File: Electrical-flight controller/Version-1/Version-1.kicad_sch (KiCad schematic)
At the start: 4 parts, among them U1 MPU-6050, U2 ATmega328P-A, U3 BMP280, U4 LM1117DT-ADJ

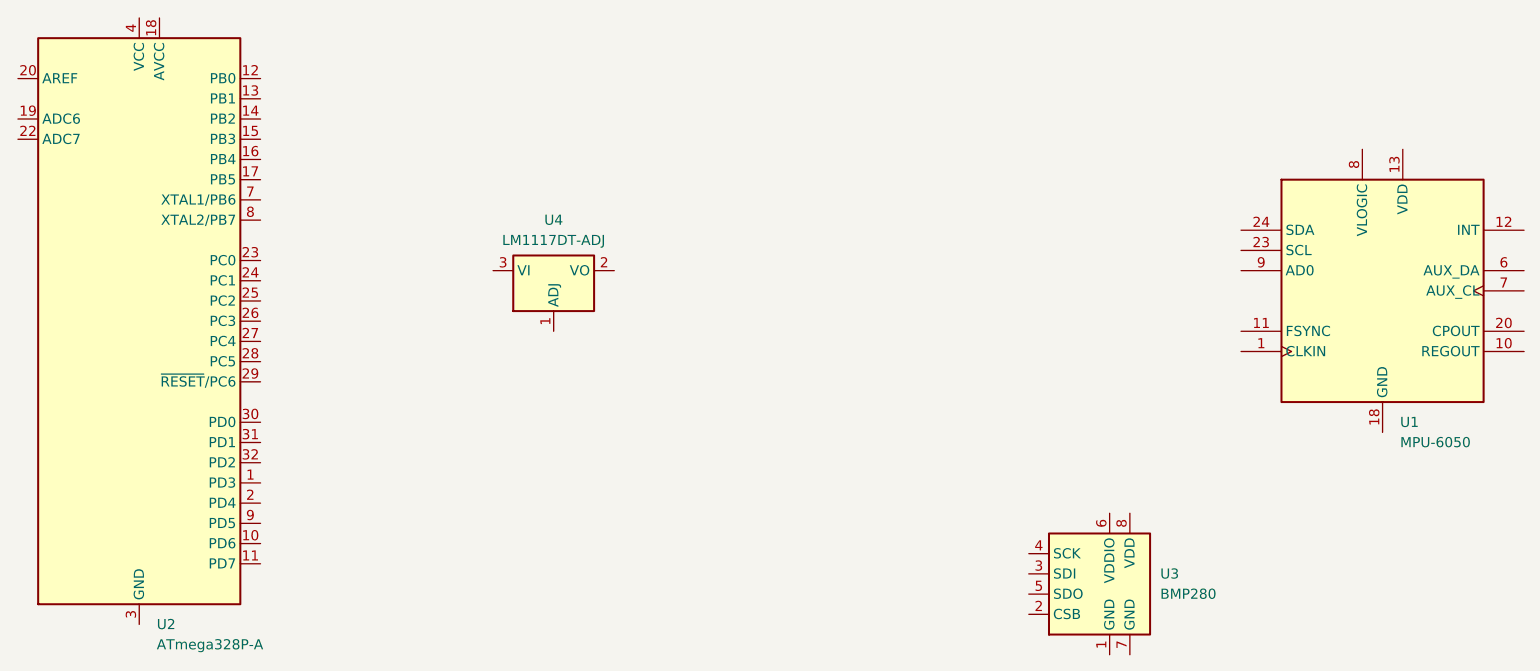
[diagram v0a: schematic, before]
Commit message: Started ESP32
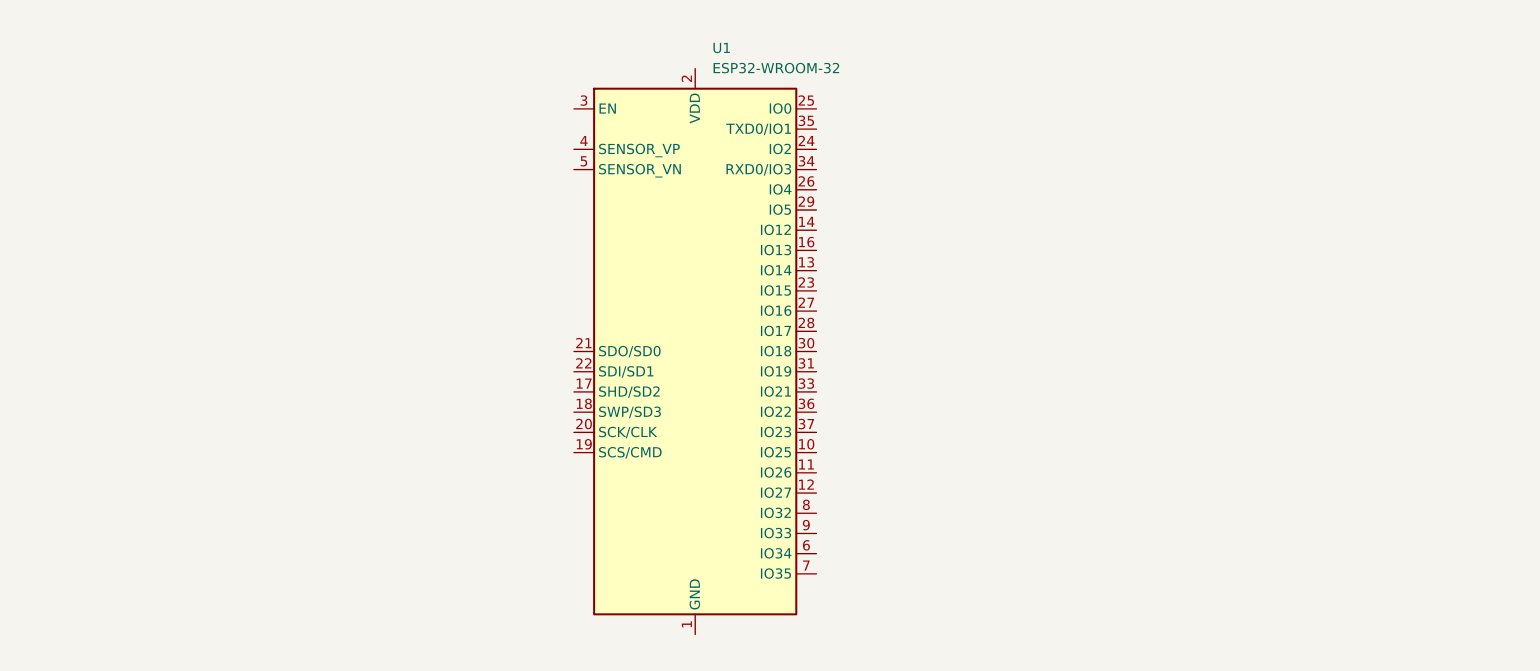
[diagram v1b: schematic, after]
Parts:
- removed U1: MPU-6050, Sensor_Motion:InvenSense_QFN-24_4x4mm_P0.5mm, symbol Sensor_Motion:MPU-6050
- removed U2: ATmega328P-A, Package_QFP:TQFP-32_7x7mm_P0.8mm, symbol MCU_Microchip_ATmega:ATmega328P-A
- removed U3: BMP280, Package_LGA:Bosch_LGA-8_2x2.5mm_P0.65mm_ClockwisePinNumbering, symbol Sensor_Pressure:BMP280
- removed U4: LM1117DT-ADJ, Package_TO_SOT_SMD:TO-252-3_TabPin2, symbol Regulator_Linear:LM1117DT-ADJ
- added U1: ESP32-WROOM-32, RF_Module:ESP32-WROOM-32, symbol RF_Module:ESP32-WROOM-32
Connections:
- new net: U1.1 (GND), U1.15 (GND), U1.38 (GND), U1.39 (GND)

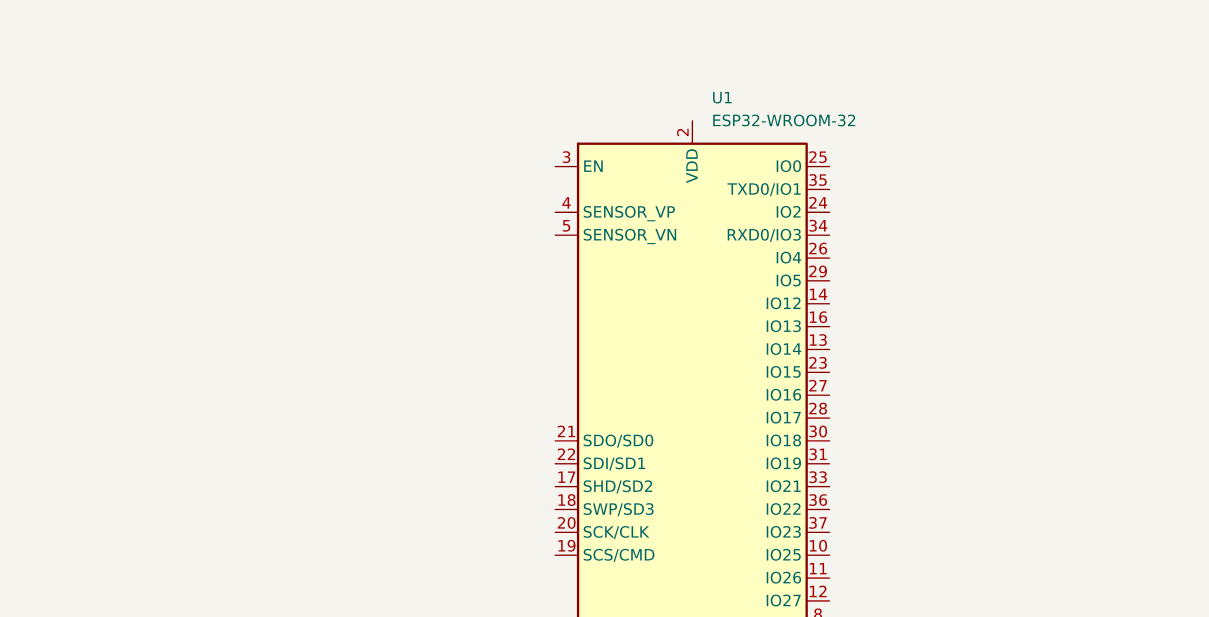
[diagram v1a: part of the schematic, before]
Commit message: 2nd update
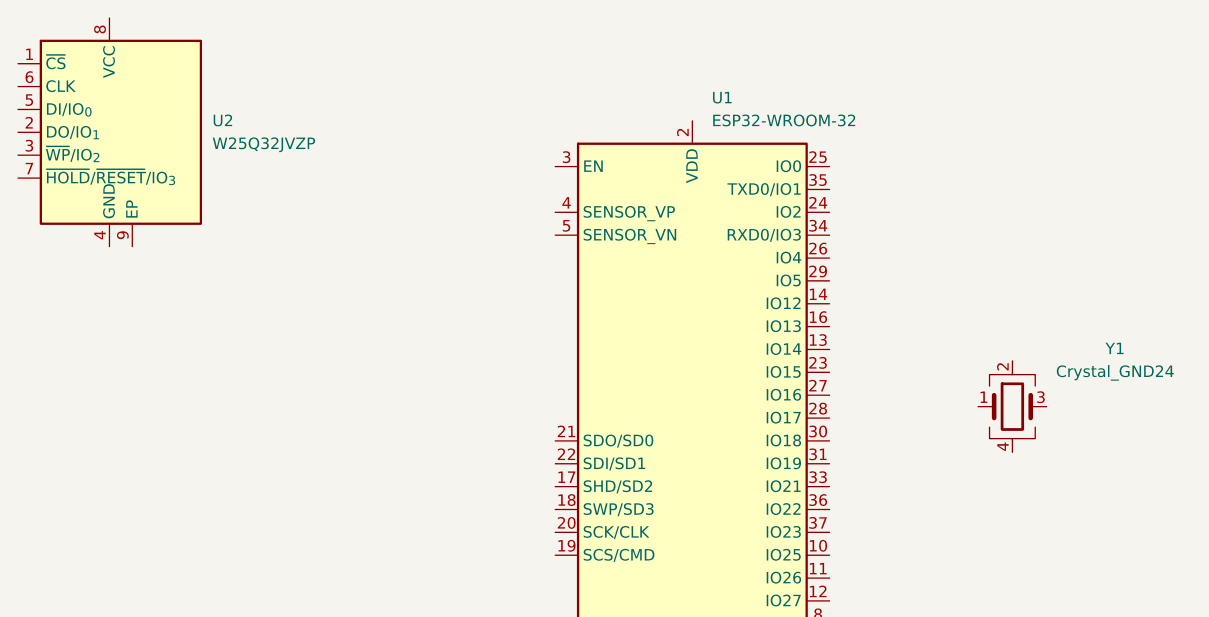
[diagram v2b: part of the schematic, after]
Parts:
- added U2: W25Q32JVZP, Package_SON:WSON-8-1EP_6x5mm_P1.27mm_EP3.4x4.3mm, symbol Memory_Flash:W25Q32JVZP
- added Y1: Crystal_GND24, symbol Device:Crystal_GND24
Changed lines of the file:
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@@
 	(paper "A4")
+	(symbol
+		(lib_id "Device:Crystal_GND24")
+		(at 170.18 78.74 0)
+		(unit 1)
+		(exclude_from_sim no)
+		(in_bom yes)
+		(on_board yes)
+		(dnp no)
+		(fields_autoplaced yes)
+		(property "Reference" "Y1"
+			(at 181.61 72.3198 0)
+			(effects
+				(font
+					(size 1.27 1.27)
+				)
+			)
+		)
+		(property "Value" "Crystal_GND24"
+			(at 181.61 74.8598 0)
+			(effects
+				(font
+					(size 1.27 1.27)
+				)
+			)
+		)
+		(property "Footprint" ""
+			(at 170.18 78.74 0)
+			(effects
+				(font
+					(size 1.27 1.27)
+				)
+				(hide yes)
+			)
+		)
+		(property "Datasheet" "~"
+			(at 170.18 78.74 0)
+			(effects
+				(font
+					(size 1.27 1.27)
+				)
+				(hide yes)
+			)
+		)
+		(property "Description" "Four pin crystal, GND on pins 2 and 4"
+			(at 170.18 78.74 0)
+			(effects
+				(font
+					(size 1.27 1.27)
+				)
+				(hide yes)
+			)
+		)
+		(pin "1"
+		)
+		(pin "2"
+		)
+		(pin "3"
+		)
+		(pin "4"
+		)
+		(instances
+			(project ""
+				(path "/b01821f6-bde1-4035-92df-fac2c021cb26"
+					(reference "Y1")
+					(unit 1)
+				)
+			)
+		)
+	)
+	(symbol
+		(lib_id "Memory_Flash:W25Q32JVZP")
+		(at 69.85 48.26 0)
+		(unit 1)
+		(exclude_from_sim no)
+		(in_bom yes)
+		(on_board yes)
+		(dnp no)
+		(fields_autoplaced yes)
+		(property "Reference" "U2"
+			(at 81.28 46.9899 0)
+			(effects
+				(font
+					(size 1.27 1.27)
+				)
+				(justify left)
+			)
+		)
+		(property "Value" "W25Q32JVZP"
+			(at 81.28 49.5299 0)
+			(effects
+				(font
+					(size 1.27 1.27)
+				)
+				(justify left)
+			)
+		)
+		(property "Footprint" "Package_SON:WSON-8-1EP_6x5mm_P1.27mm_EP3.4x4.3mm"
+			(at 69.85 48.26 0)
+			(effects
+				(font
+					(size 1.27 1.27)
+				)
+				(hide yes)
+			)
+		)
+		(property "Datasheet" "http://www.winbond.com/resource-files/w25q32jv%20revg%2003272018%20plus.pdf"
+			(at 69.85 50.8 0)
+			(effects
+				(font
+					(size 1.27 1.27)
+				)
+				(hide yes)
+			)
+		)
+		(property "Description" "32Mbit / 4MiB Serial Flash Memory, Standard/Dual/Quad SPI, 2.7-3.6V, WSON-8"
+			(at 69.85 48.26 0)
+			(effects
+				(font
+					(size 1.27 1.27)
+				)
+				(hide yes)
+			)
+		)
+		(pin "5"
+		)
+		(pin "7"
+		)
+		(pin "2"
+		)
+		(pin "9"
+		)
+		(pin "1"
+		)
+		(pin "6"
+		)
+		(pin "3"
+		)
+		(pin "8"
+		)
+		(pin "4"
+		)
+		(instances
+			(project ""
+				(path "/b01821f6-bde1-4035-92df-fac2c021cb26"
+					(reference "U2")
+					(unit 1)
+				)
+			)
+		)
+	)
 	(symbol
 		(lib_id "RF_Module:ESP32-WROOM-32")

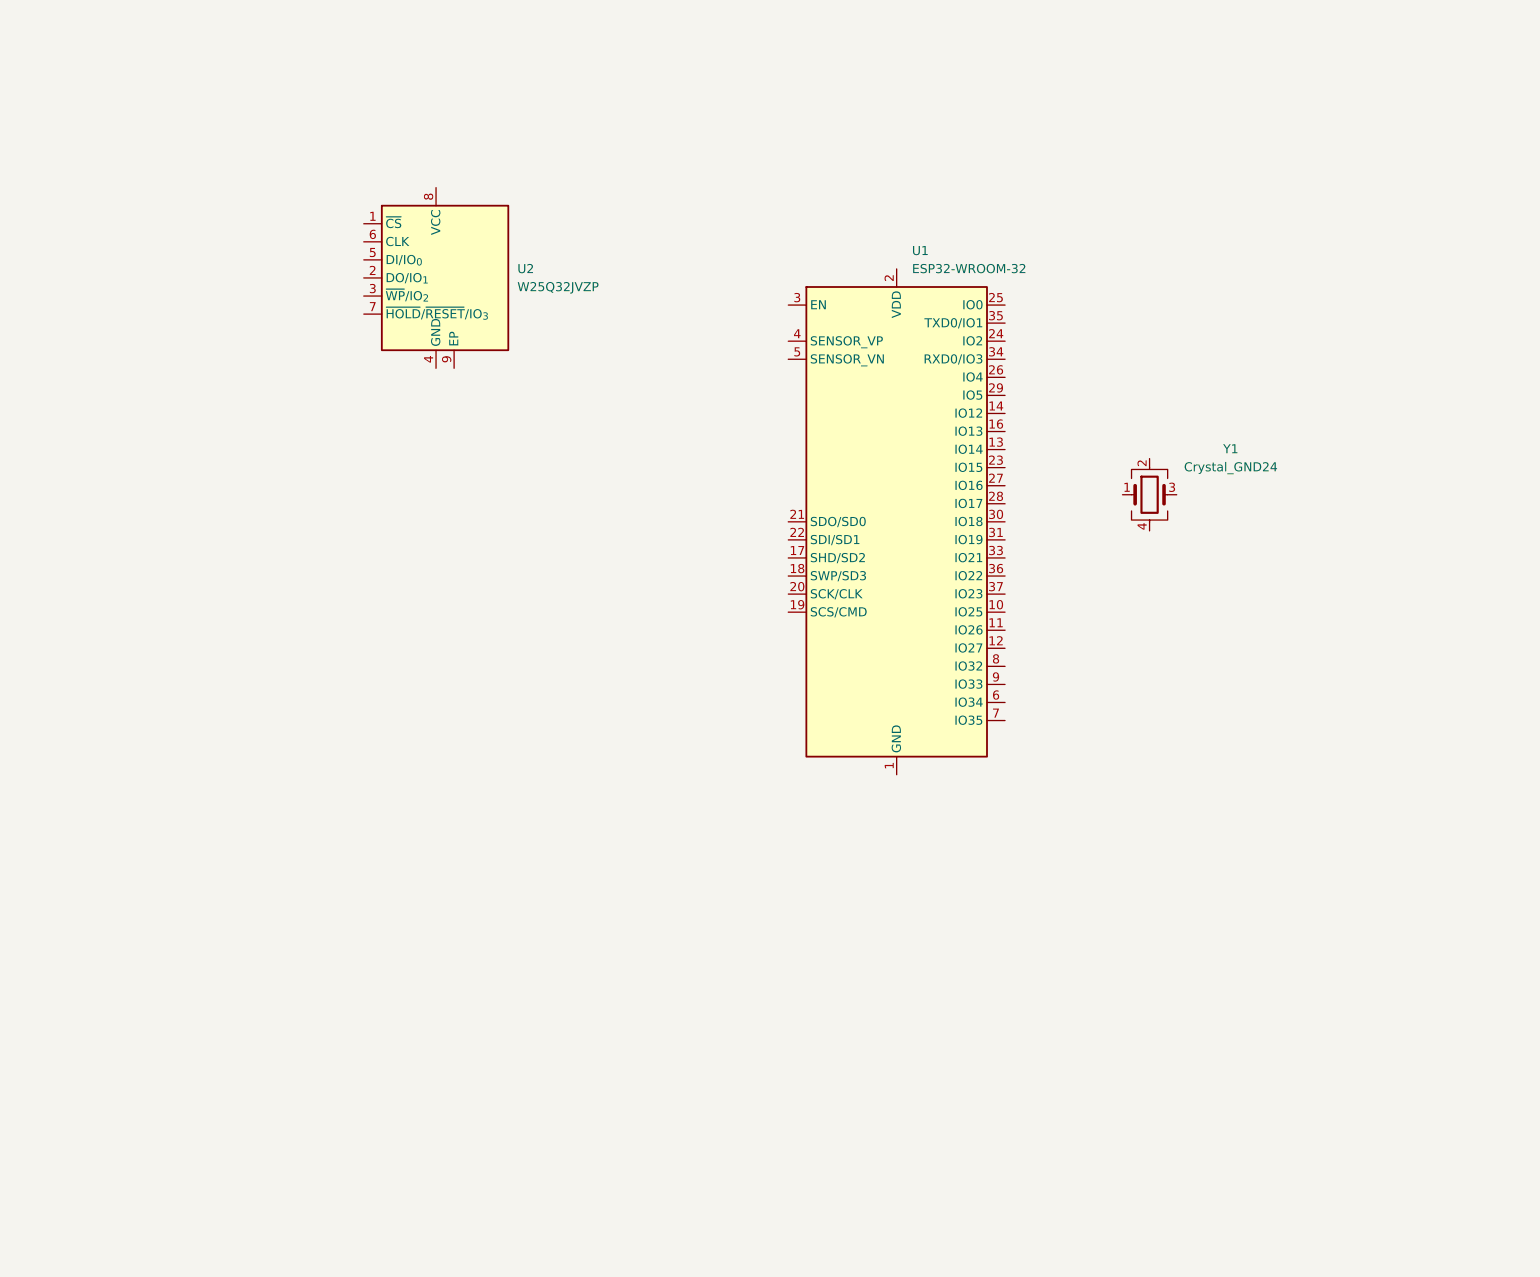
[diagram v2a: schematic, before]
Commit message: power circuit
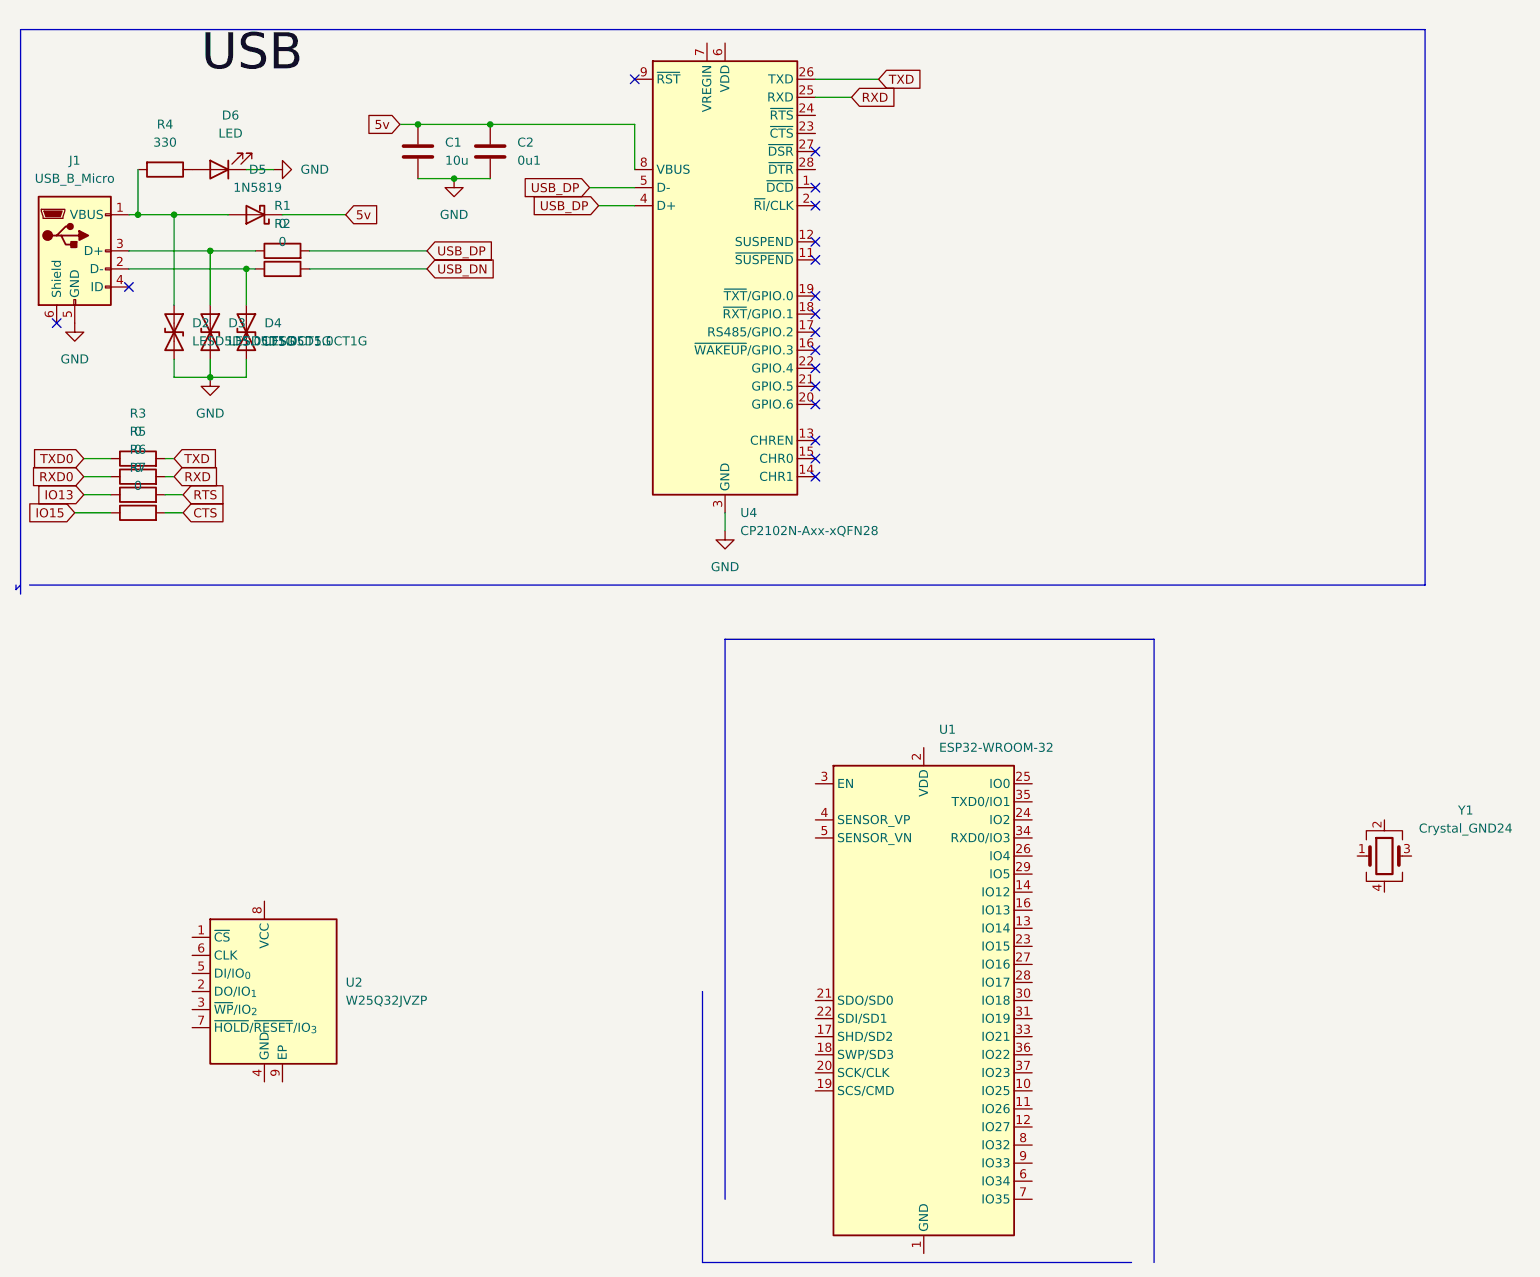
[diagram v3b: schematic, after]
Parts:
- added C1: 10u, symbol Device:C
- added C2: 0u1, symbol Device:C
- added D2, D3, D4: LESD5D5.0CT1G, symbol Device:D_TVS
- added D5: 1N5819, Diode_THT:D_DO-41_SOD81_P10.16mm_Horizontal, symbol Diode:1N5819
- added D6: LED, LED_SMD:LED_0201_0603Metric, symbol Device:LED
- added J1: USB_B_Micro, symbol Connector:USB_B_Micro
- added R1, R2, R3, R5, R6, R7: 0, symbol Device:R
- added R4: 330, Resistor_SMD:R_0402_1005Metric, symbol Device:R
- added U4: CP2102N-Axx-xQFN28, Package_DFN_QFN:QFN-28-1EP_5x5mm_P0.5mm_EP3.35x3.35mm, symbol Interface_USB:CP2102N-Axx-xQFN28
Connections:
- new net: D6.2 (A), R4.1
- new net: D3.1 (A1), J1.3 (D+), R1.1
- new net: D4.1 (A1), J1.2 (D-), R2.1
- new net: D2.1 (A1), D5.2 (A), J1.1 (VBUS), R4.2
- new net 5v: C1.1, C2.1, D5.1 (K), U4.8 (VBUS)
- new net CTS: R7.2
- new net GND: C1.2, C2.2, D2.2 (A2), D3.2 (A2), D4.2 (A2), D6.1 (K), J1.5 (GND), U4.29 (GND), U4.3 (GND)
- new net IO13: R6.1
- new net IO15: R7.1
- new net RTS: R6.2
- new net RXD: R5.2, U4.25 (RXD)
- new net RXD0: R5.1
- new net TXD: R3.2, U4.26 (TXD)
- new net TXD0: R3.1
- new net USB_DN: R2.2
- new net USB_DP: R1.2, U4.4 (D+), U4.5 (D-)
- no-connect marks 0 -> 18
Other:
- moved on the sheet: U1, U2, Y1
